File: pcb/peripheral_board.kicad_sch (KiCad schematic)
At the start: 2 parts

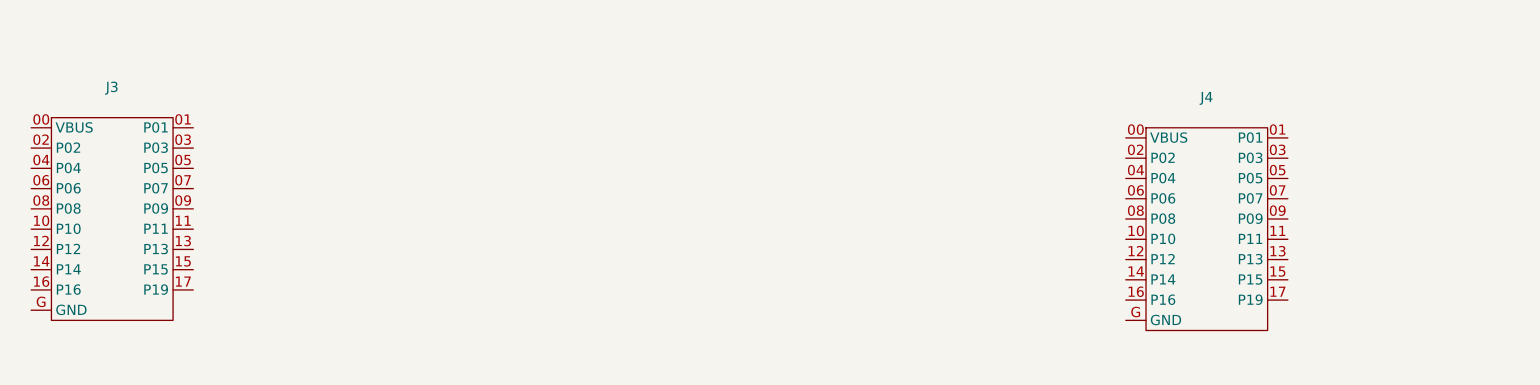
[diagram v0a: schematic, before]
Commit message: Continue work on PCBs.
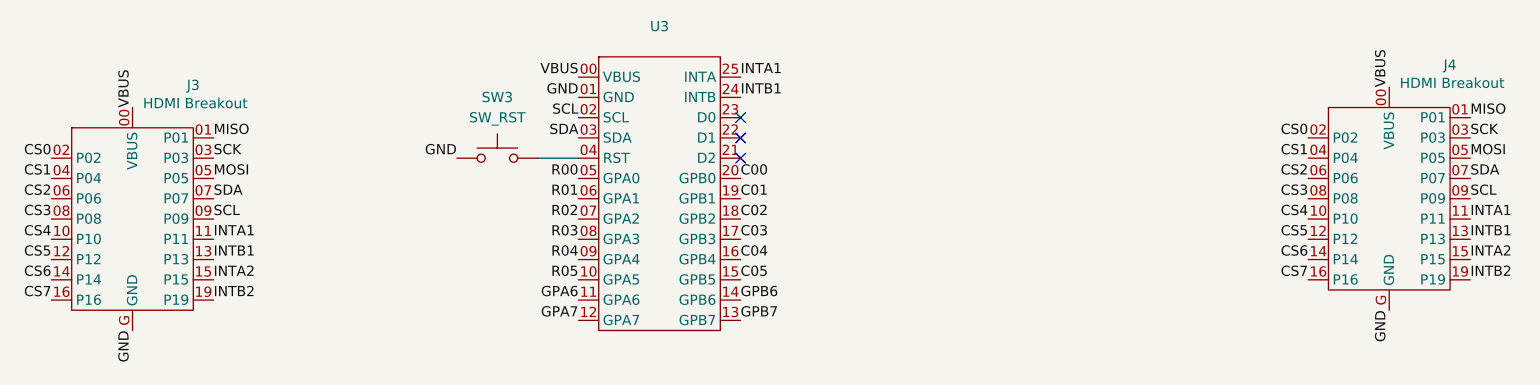
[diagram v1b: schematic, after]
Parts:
- added SW3: SW_RST, Button_Switch_THT:SW_PUSH_6mm, symbol Switch:SW_Push
- added U3: ~, excelsior:MCP23017_Breakout, symbol excelsior:MCP23017_Breakout
- J3, J4: value ~ -> HDMI Breakout
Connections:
- net VBUS: now reaches J4.00 (VBUS)
- net VBUS: now also J3.00 (VBUS), U3.00 (VBUS)
- net MISO: now reaches J4.01 (P01)
- net MISO: now also J3.01 (P01)
- net CS0: now reaches J4.02 (P02)
- net CS0: now also J3.02 (P02)
- net SCK: now reaches J4.03 (P03)
- net SCK: now also J3.03 (P03)
- net CS1: now reaches J4.04 (P04)
- net CS1: now also J3.04 (P04)
- net MOSI: now reaches J4.05 (P05)
- net MOSI: now also J3.05 (P05)
- net CS2: now reaches J4.06 (P06)
- net CS2: now also J3.06 (P06)
- net SDA: now reaches J4.07 (P07)
- net SDA: now also J3.07 (P07), U3.03 (SDA)
- net CS3: now reaches J4.08 (P08)
- net CS3: now also J3.08 (P08)
- net SCL: now reaches J4.09 (P09)
- net SCL: now also J3.09 (P09), U3.02 (SCL)
- net CS4: now reaches J4.10 (P10)
- net CS4: now also J3.10 (P10)
- net INTA1: now reaches J4.11 (P11)
- net INTA1: now also J3.11 (P11), U3.25 (INTA)
- net CS5: now reaches J4.12 (P12)
- net CS5: now also J3.12 (P12)
- net INTB1: now reaches J4.13 (P13)
- net INTB1: now also J3.13 (P13), U3.24 (INTB)
- net CS6: now reaches J4.14 (P14)
- net CS6: now also J3.14 (P14)
- net INTA2: now reaches J4.15 (P15)
- net INTA2: now also J3.15 (P15)
- net CS7: now reaches J4.16 (P16)
- net CS7: now also J3.16 (P16)
- net GND: now reaches J4.G (GND)
- net GND: now also J3.G (GND), SW3.1, U3.01 (GND)
- new net: SW3.2, U3.04 (RST)
- new net C00: U3.20 (GPB0)
- new net C01: U3.19 (GPB1)
- new net C02: U3.18 (GPB2)
- new net C03: U3.17 (GPB3)
- new net C04: U3.16 (GPB4)
- new net C05: U3.15 (GPB5)
- new net GPA6: U3.11 (GPA6)
- new net GPA7: U3.12 (GPA7)
- new net GPB6: U3.14 (GPB6)
- new net GPB7: U3.13 (GPB7)
- new net INTB2: J3.19 (P19), J4.19 (P19)
- new net R00: U3.05 (GPA0)
- new net R01: U3.06 (GPA1)
- new net R02: U3.07 (GPA2)
- new net R03: U3.08 (GPA3)
- new net R04: U3.09 (GPA4)
- new net R05: U3.10 (GPA5)
- no-connect marks 0 -> 3
